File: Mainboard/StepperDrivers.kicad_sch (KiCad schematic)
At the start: 9 parts

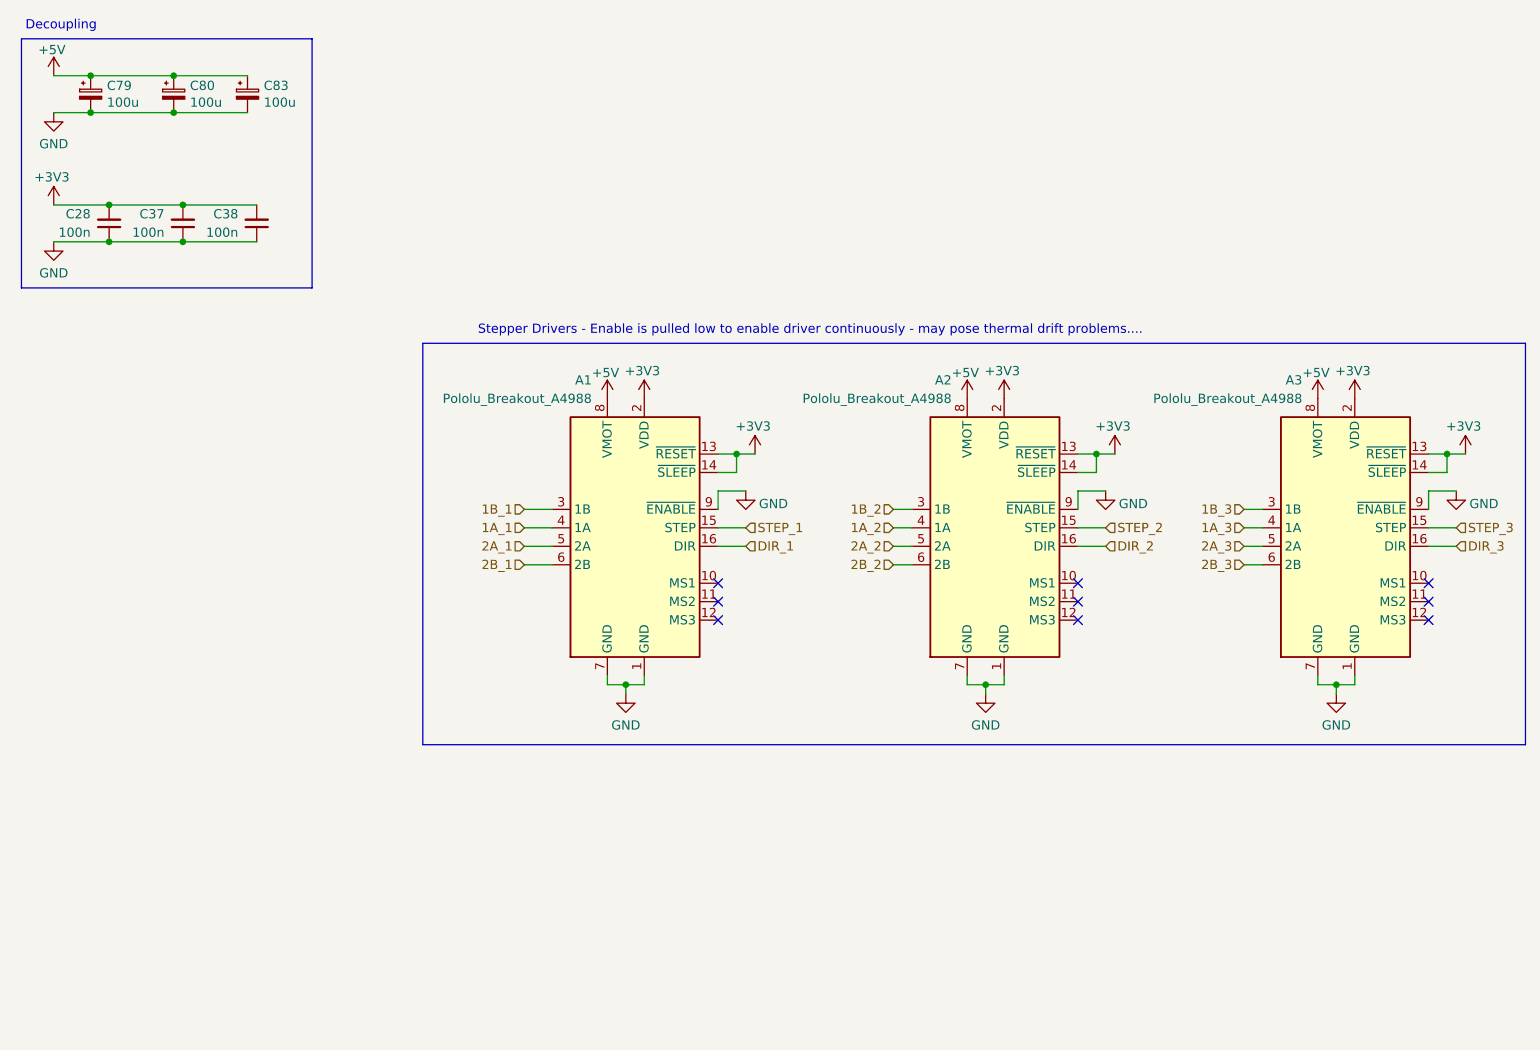
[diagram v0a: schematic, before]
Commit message: cad update
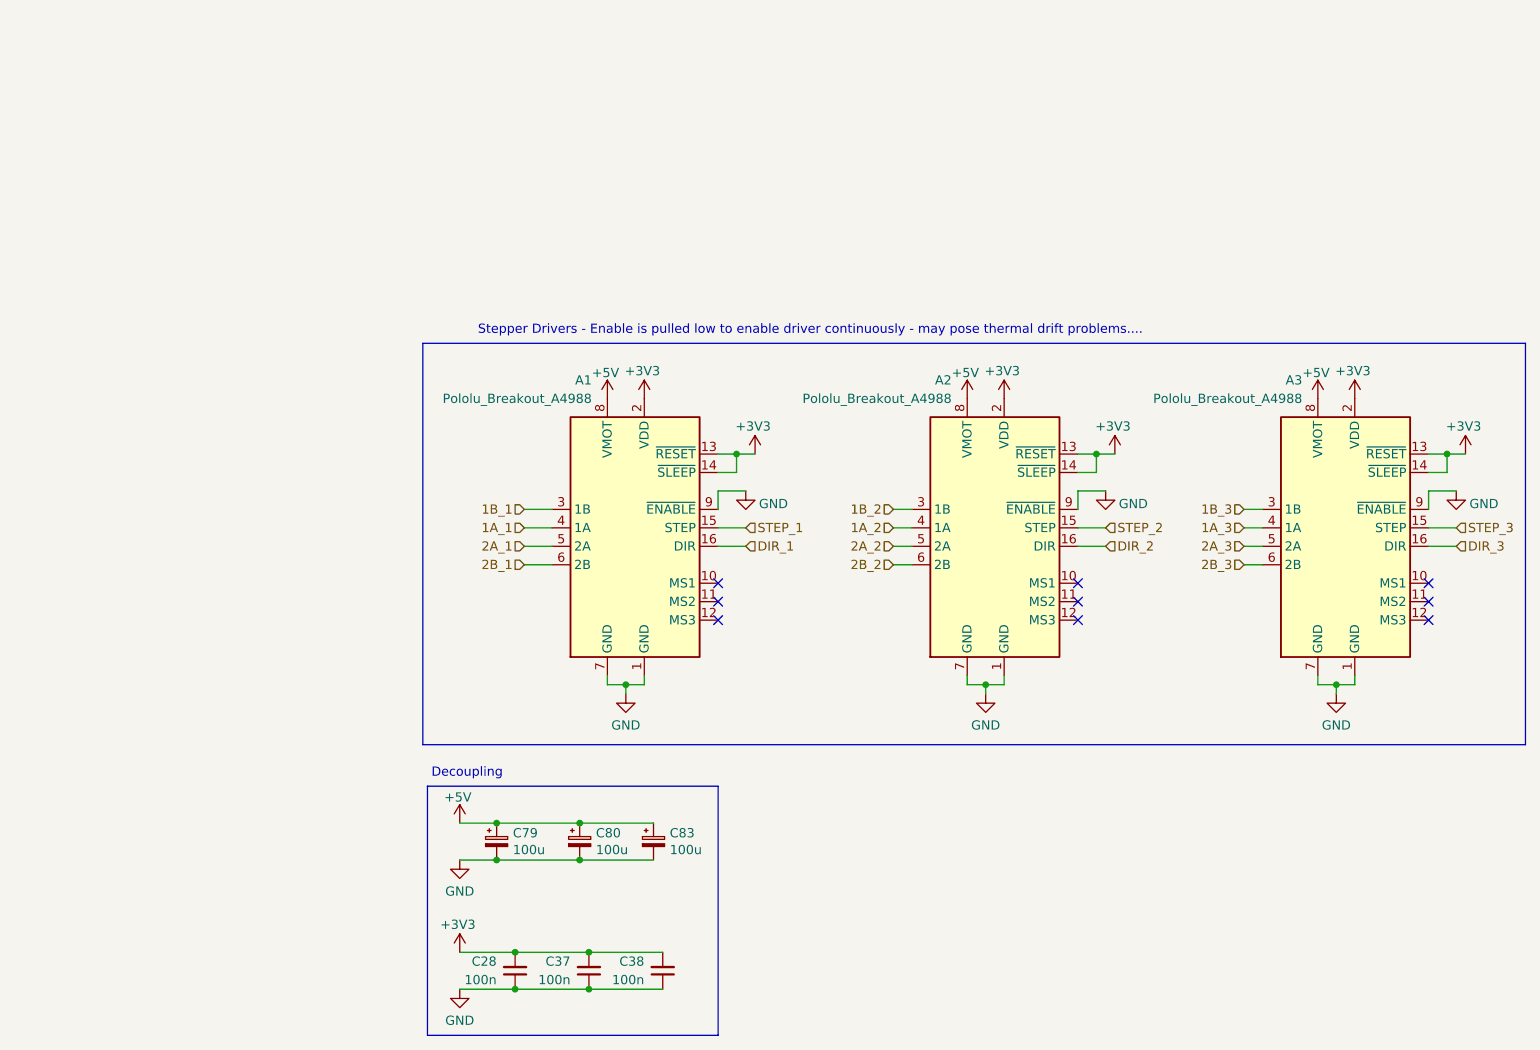
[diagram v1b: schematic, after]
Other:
- moved on the sheet: C28, C37, C38, C79, C80, C83
